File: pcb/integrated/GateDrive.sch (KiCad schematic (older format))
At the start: 14 parts, among them U11001 UCC5350SB, U11002 R15P21503D

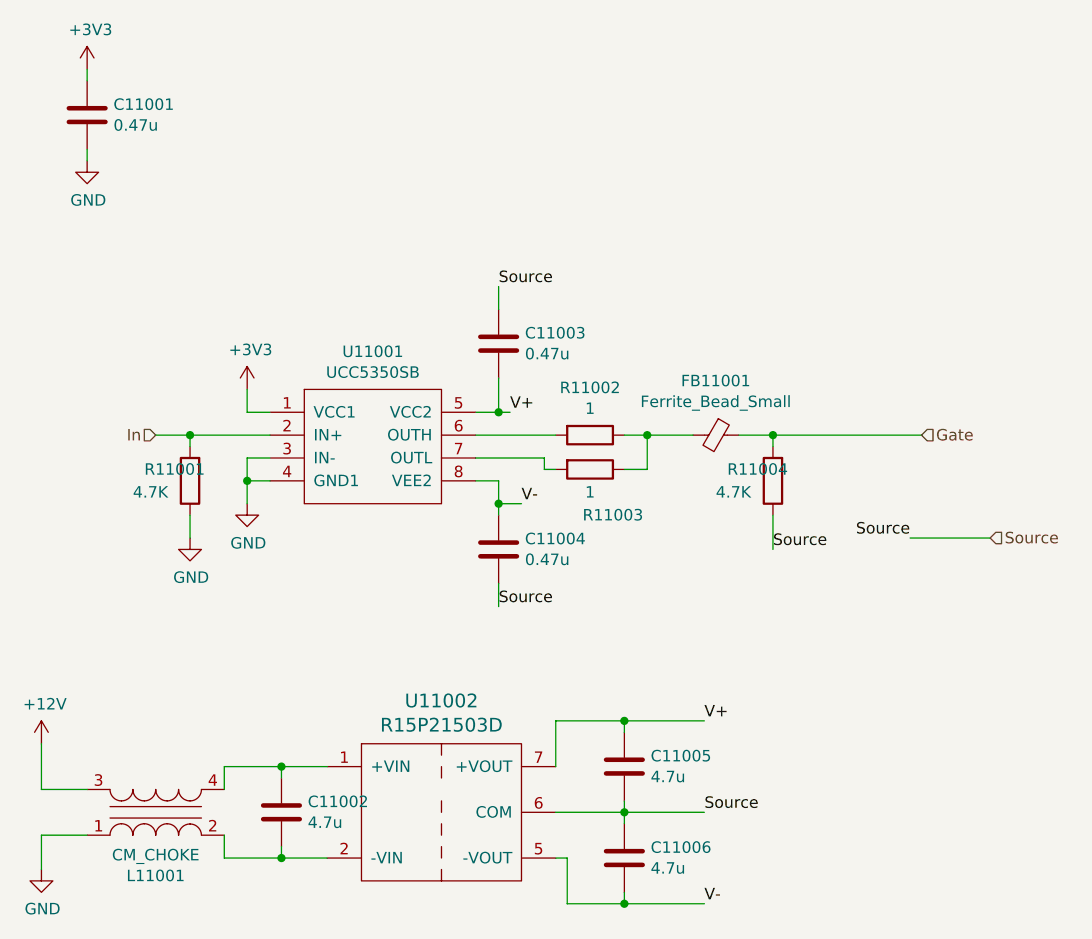
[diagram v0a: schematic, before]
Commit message: PCB routing finihsed, ready for design review
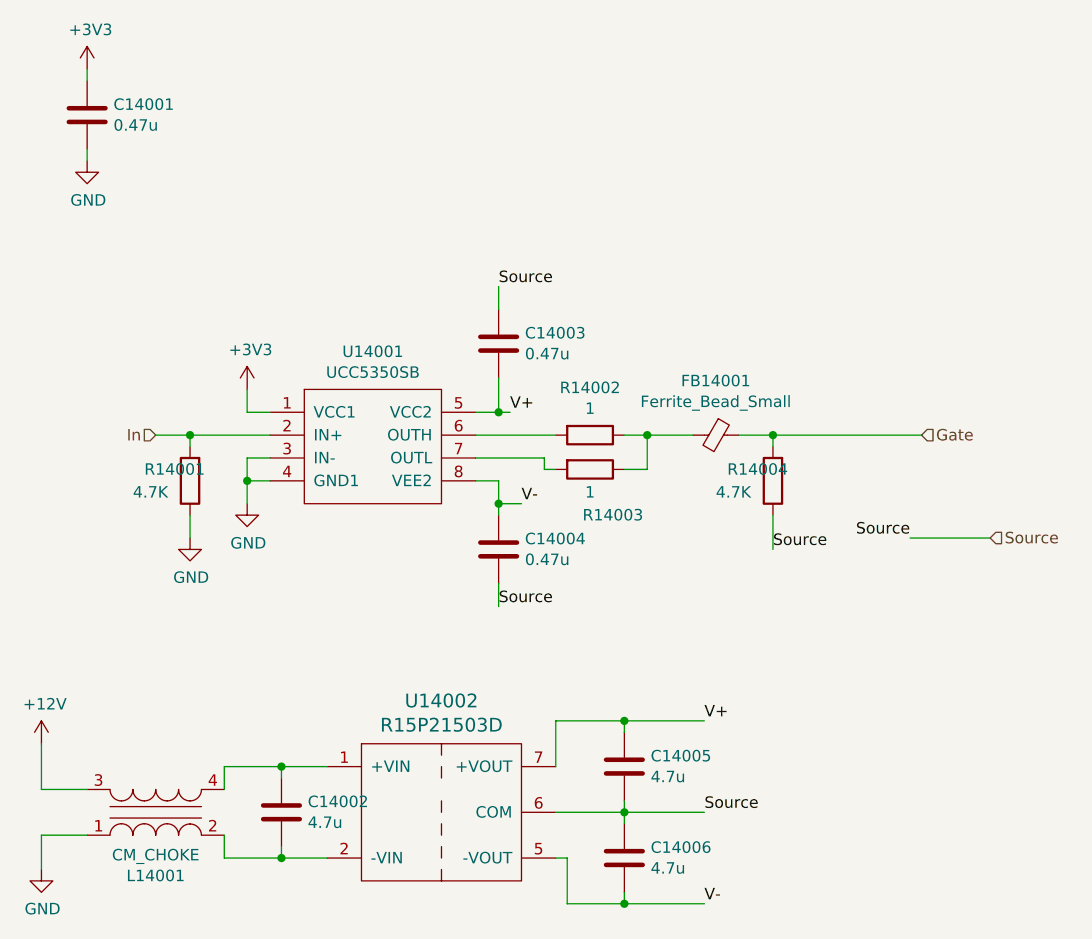
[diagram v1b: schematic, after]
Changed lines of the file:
@@
 AR Path="/5D68A538/5D640674/5DD374B5" Ref="U13002"  Part="1"
 AR Path="/5D68A538/5D640682/5DD374B5" Ref="U14002"  Part="1"
-F 0 "U11002" H 3450 5237 60  0000 C CNN
+F 0 "U14002" H 3450 5237 60  0000 C CNN
 F 1 "R15P21503D" H 3450 5131 60  0000 C CNN
 F 2 "wbraun_smd:SIP7-5" H 3450 4850 60  0001 C CNN
@@
 AR Path="/5D68A538/5D640674/5DD374B6" Ref="U13001"  Part="1"
 AR Path="/5D68A538/5D640682/5DD374B6" Ref="U14001"  Part="1"
-F 0 "U11001" H 3150 3565 50  0000 C CNN
+F 0 "U14001" H 3150 3565 50  0000 C CNN
 F 1 "UCC5350SB" H 3150 3474 50  0000 C CNN
 F 2 "Package_SO:SOIC-8_3.9x4.9mm_P1.27mm" H 2800 3200 50  0001 C CNN
@@
 AR Path="/5D68A538/5D640674/5DD374B7" Ref="C13002"  Part="1"
 AR Path="/5D68A538/5D640682/5DD374B7" Ref="C14002"  Part="1"
-F 0 "C11002" H 2865 4796 50  0000 L CNN
+F 0 "C14002" H 2865 4796 50  0000 L CNN
 F 1 "4.7u" H 2865 4705 50  0000 L CNN
 F 2 "Capacitor_SMD:C_0805_2012Metric" H 2788 4600 50  0001 C CNN
@@
 AR Path="/5D68A538/5D640674/5D630902" Ref="C13005"  Part="1"
 AR Path="/5D68A538/5D640682/5D630902" Ref="C14005"  Part="1"
-F 0 "C11005" H 4365 4596 50  0000 L CNN
+F 0 "C14005" H 4365 4596 50  0000 L CNN
 F 1 "4.7u" H 4365 4505 50  0000 L CNN
 F 2 "Capacitor_SMD:C_0805_2012Metric" H 4288 4400 50  0001 C CNN
@@
 AR Path="/5D68A538/5D640674/5D630909" Ref="C13006"  Part="1"
 AR Path="/5D68A538/5D640682/5D630909" Ref="C14006"  Part="1"
-F 0 "C11006" H 4365 4996 50  0000 L CNN
+F 0 "C14006" H 4365 4996 50  0000 L CNN
 F 1 "4.7u" H 4365 4905 50  0000 L CNN
 F 2 "Capacitor_SMD:C_0805_2012Metric" H 4288 4800 50  0001 C CNN
@@
 AR Path="/5D68A538/5D640674/5D630910" Ref="C13003"  Part="1"
 AR Path="/5D68A538/5D640682/5D630910" Ref="C14003"  Part="1"
-F 0 "C11003" H 3815 2746 50  0000 L CNN
+F 0 "C14003" H 3815 2746 50  0000 L CNN
 F 1 "0.47u" H 3815 2655 50  0000 L CNN
 F 2 "Capacitor_SMD:C_0603_1608Metric" H 3738 2550 50  0001 C CNN
@@
 AR Path="/5D68A538/5D640674/5DD374BB" Ref="C13004"  Part="1"
 AR Path="/5D68A538/5D640682/5DD374BB" Ref="C14004"  Part="1"
-F 0 "C11004" H 3815 3646 50  0000 L CNN
+F 0 "C14004" H 3815 3646 50  0000 L CNN
 F 1 "0.47u" H 3815 3555 50  0000 L CNN
 F 2 "Capacitor_SMD:C_0603_1608Metric" H 3738 3450 50  0001 C CNN
@@
 AR Path="/5D68A538/5D640674/5D63091E" Ref="R13002"  Part="1"
 AR Path="/5D68A538/5D640682/5D63091E" Ref="R14002"  Part="1"
-F 0 "R11002" V 3893 3100 50  0000 C CNN
+F 0 "R14002" V 3893 3100 50  0000 C CNN
 F 1 "1" V 3984 3100 50  0000 C CNN
 F 2 "Resistor_SMD:R_0805_2012Metric" V 4030 3100 50  0001 C CNN
@@
 AR Path="/5D68A538/5D640674/5D630925" Ref="R13003"  Part="1"
 AR Path="/5D68A538/5D640682/5D630925" Ref="R14003"  Part="1"
-F 0 "R11003" V 4300 3350 50  0000 C CNN
+F 0 "R14003" V 4300 3350 50  0000 C CNN
 F 1 "1" V 4200 3250 50  0000 C CNN
 F 2 "Resistor_SMD:R_0805_2012Metric" V 4030 3250 50  0001 C CNN
@@
 AR Path="/5D68A538/5D640674/5D63094B" Ref="R13001"  Part="1"
 AR Path="/5D68A538/5D640682/5D63094B" Ref="R14001"  Part="1"
-F 0 "R11001" H 2550 3250 50  0000 R CNN
+F 0 "R14001" H 2550 3250 50  0000 R CNN
 F 1 "4.7K" H 2600 3350 50  0000 R CNN
 F 2 "Resistor_SMD:R_0603_1608Metric" V 2280 3300 50  0001 C CNN
@@
 AR Path="/5D68A538/5D640674/5D630960" Ref="C13001"  Part="1"
 AR Path="/5D68A538/5D640682/5D630960" Ref="C14001"  Part="1"
-F 0 "C11001" H 2015 1746 50  0000 L CNN
+F 0 "C14001" H 2015 1746 50  0000 L CNN
 F 1 "0.47u" H 2015 1655 50  0000 L CNN
 F 2 "Capacitor_SMD:C_0603_1608Metric" H 1938 1550 50  0001 C CNN
@@
 AR Path="/5D68A538/5D640674/5D63A672" Ref="FB13001"  Part="1"
 AR Path="/5D68A538/5D640682/5D63A672" Ref="FB14001"  Part="1"
-F 0 "FB11001" V 4413 3100 50  0000 C CNN
+F 0 "FB14001" V 4413 3100 50  0000 C CNN
 F 1 "Ferrite_Bead_Small" V 4504 3100 50  0000 C CNN
 F 2 "Inductor_SMD:L_0805_2012Metric" V 4580 3100 50  0001 C CNN
@@
 AR Path="/5D68A538/5D640674/5DD374C9" Ref="R13004"  Part="1"
 AR Path="/5D68A538/5D640682/5DD374C9" Ref="R14004"  Part="1"
-F 0 "R11004" H 5100 3250 50  0000 R CNN
+F 0 "R14004" H 5100 3250 50  0000 R CNN
 F 1 "4.7K" H 5150 3350 50  0000 R CNN
 F 2 "Resistor_SMD:R_0603_1608Metric" V 4830 3300 50  0001 C CNN
@@
 AR Path="/5D68A538/5D640674/5D63092C" Ref="L13001"  Part="1"
 AR Path="/5D68A538/5D640682/5D63092C" Ref="L14001"  Part="1"
-F 0 "L11001" H 2200 5028 50  0000 C CNN
+F 0 "L14001" H 2200 5028 50  0000 C CNN
 F 1 "CM_CHOKE" H 2200 4937 50  0000 C CNN
 F 2 "wbraun_smd:SRF2012" V 2200 4750 50  0001 C CNN
